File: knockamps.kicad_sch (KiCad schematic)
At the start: 6 parts, among them M6001 Module-knock-0.2, M6002 Module-knock-0.2, U6001 MCP6002-xSN

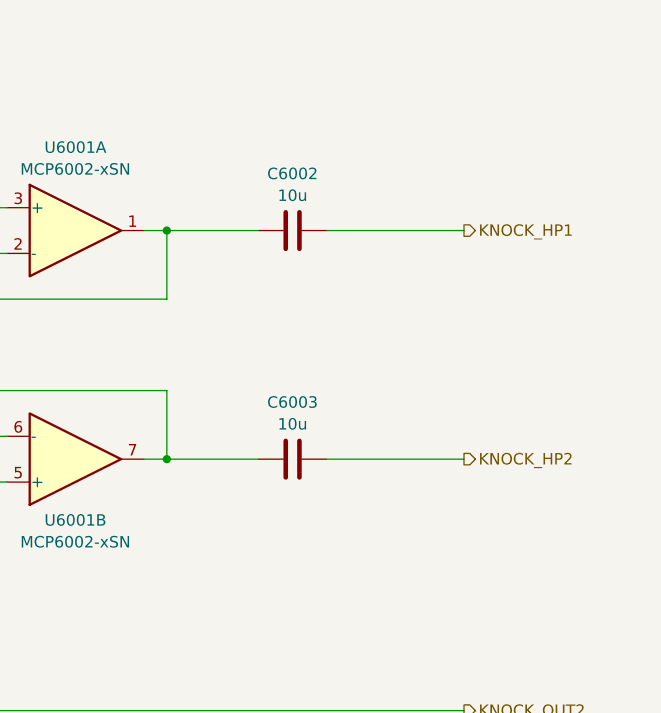
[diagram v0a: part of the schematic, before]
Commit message: Initial schematic
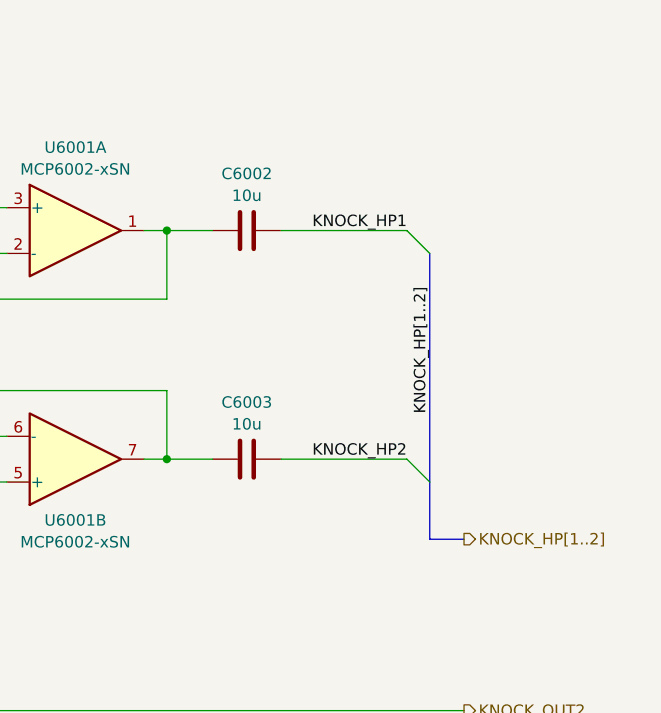
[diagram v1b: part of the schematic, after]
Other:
- moved on the sheet: C6002, C6003
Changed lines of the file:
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@@
+		)
+	)
+	(bus_entry
+		(at 240.03 99.06)
+		(size 2.54 2.54)
+		(stroke
+			(width 0)
+			(type default)
+		)
+	)
+	(bus_entry
+		(at 240.03 73.66)
+		(size 2.54 2.54)
+		(stroke
+			(width 0)
+			(type default)
 		)
 	)
@@
 	(wire
 		(pts
-			(xy 213.36 99.06) (xy 223.52 99.06)
+			(xy 213.36 99.06) (xy 218.44 99.06)
 		)
 		(stroke
@@
 	(wire
 		(pts
+			(xy 226.06 73.66) (xy 240.03 73.66)
+		)
+		(stroke
+			(width 0)
+			(type default)
+		)
+	)
+	(wire
+		(pts
 			(xy 138.43 97.79) (xy 138.43 21.59)
 		)
@@
 	(wire
 		(pts
-			(xy 231.14 99.06) (xy 246.38 99.06)
-		)
-		(stroke
-			(width 0)
-			(type default)
-		)
-	)
-	(wire
-		(pts
 			(xy 58.42 45.72) (xy 72.39 45.72)
 		)
@@
 		)
 	)
-	(wire
-		(pts
-			(xy 231.14 73.66) (xy 246.38 73.66)
+	(bus
+		(pts
+			(xy 246.38 107.95) (xy 242.57 107.95)
 		)
 		(stroke
@@
 		)
 	)
+	(bus
+		(pts
+			(xy 242.57 76.2) (xy 242.57 101.6)
+		)
+		(stroke
+			(width 0)
+			(type default)
+		)
+	)
 	(wire
 		(pts
@@
 	(wire
 		(pts
+			(xy 226.06 99.06) (xy 240.03 99.06)
+		)
+		(stroke
+			(width 0)
+			(type default)
+		)
+	)
+	(wire
+		(pts
 			(xy 153.67 76.2) (xy 163.83 76.2)
 		)
@@
 		)
 	)
+	(bus
+		(pts
+			(xy 242.57 107.95) (xy 242.57 101.6)
+		)
+		(stroke
+			(width 0)
+			(type default)
+		)
+	)
 	(wire
 		(pts
@@
 	(wire
 		(pts
-			(xy 213.36 73.66) (xy 223.52 73.66)
+			(xy 213.36 73.66) (xy 218.44 73.66)
 		)
 		(stroke
@@
 			(width 0)
 			(type default)
+		)
+	)
+	(label "KNOCK_HP1"
+		(at 240.03 73.66 180)
+		(effects
+			(font
+				(size 1.27 1.27)
+			)
+			(justify right bottom)
 		)
 	)
@@
 		)
 	)
+	(label "KNOCK_HP2"
+		(at 240.03 99.06 180)
+		(effects
+			(font
+				(size 1.27 1.27)
+			)
+			(justify right bottom)
+		)
+	)
 	(label "KNOCK1"
 		(at 60.96 45.72 0)
+		(effects
+			(font
+				(size 1.27 1.27)
+			)
+			(justify left bottom)
+		)
+	)
+	(label "KNOCK_HP[1..2]"
+		(at 242.57 93.98 90)
 		(effects
 			(font
@@
 		)
 	)
-	(hierarchical_label "KNOCK_HP1"
+	(hierarchical_label "KNOCK_HP[1..2]"
 		(shape output)
-		(at 246.38 73.66 0)
+		(at 246.38 107.95 0)
 		(effects
 			(font
@@
 		(shape output)
 		(at 246.38 45.72 0)
-		(effects
-			(font
-				(size 1.27 1.27)
-			)
-			(justify left)
-		)
-	)
-	(hierarchical_label "KNOCK_HP2"
-		(shape output)
-		(at 246.38 99.06 0)
 		(effects
 			(font
@@
 	(symbol
 		(lib_id "Device:C")
-		(at 227.33 73.66 90)
+		(at 222.25 73.66 90)
 		(unit 1)
 		(exclude_from_sim no)
@@
 		(fields_autoplaced yes)
 		(property "Reference" "C6002"
-			(at 227.33 67.3565 90)
+			(at 222.25 67.3565 90)
 			(effects
 				(font
@@
 		)
 		(property "Value" "10u"
-			(at 227.33 69.7808 90)
+			(at 222.25 69.7808 90)
 			(effects
 				(font
@@
 		)
 		(property "Footprint" "Capacitor_SMD:C_0603_1608Metric"
-			(at 231.14 72.6948 0)
+			(at 226.06 72.6948 0)
 			(effects
 				(font
@@
 		)
 		(property "Datasheet" "~"
-			(at 227.33 73.66 0)
+			(at 222.25 73.66 0)
 			(effects
 				(font
@@
 		)
 		(property "Description" "Unpolarized capacitor"
-			(at 227.33 73.66 0)
+			(at 222.25 73.66 0)
 			(effects
 				(font
@@
 	(symbol
 		(lib_id "Device:C")
-		(at 227.33 99.06 90)
+		(at 222.25 99.06 90)
 		(unit 1)
 		(exclude_from_sim no)
@@
 		(fields_autoplaced yes)
 		(property "Reference" "C6003"
-			(at 227.33 92.7565 90)
+			(at 222.25 92.7565 90)
 			(effects
 				(font
@@
 		)
 		(property "Value" "10u"
-			(at 227.33 95.1808 90)
+			(at 222.25 95.1808 90)
 			(effects
 				(font
@@
 		)
 		(property "Footprint" "Capacitor_SMD:C_0603_1608Metric"
-			(at 231.14 98.0948 0)
+			(at 226.06 98.0948 0)
 			(effects
 				(font
@@
 		)
 		(property "Datasheet" "~"
-			(at 227.33 99.06 0)
+			(at 222.25 99.06 0)
 			(effects
 				(font
@@
 		)
 		(property "Description" "Unpolarized capacitor"
-			(at 227.33 99.06 0)
-			(effects
-				(font
+			(at 222.25 99.06 0)
+			(effects
+				(font

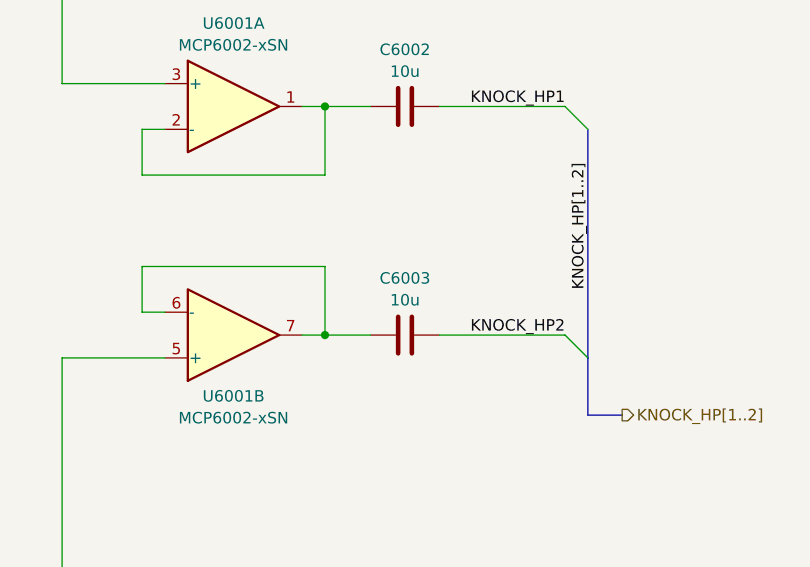
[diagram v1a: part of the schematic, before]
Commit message: adjusted BOM
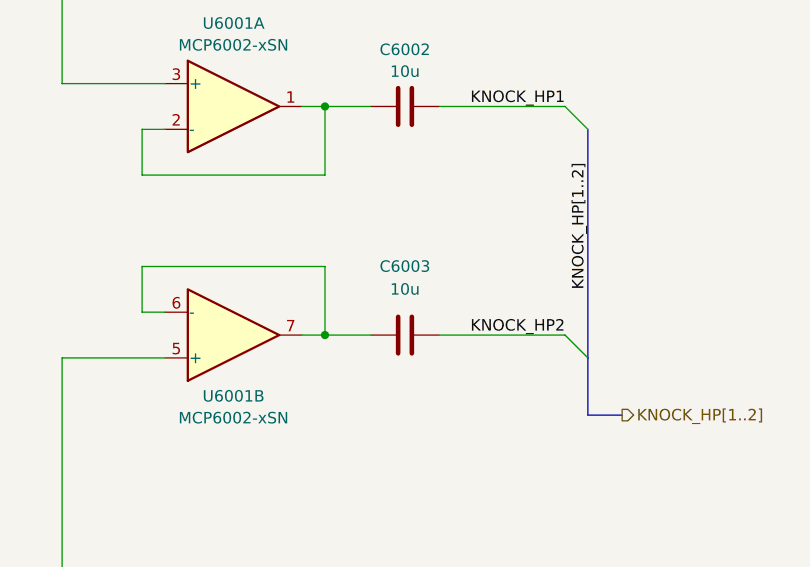
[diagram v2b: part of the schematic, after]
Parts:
- C6001: footprint Capacitor_SMD:C_0603_1608Metric -> hellen-one-common:C0805; LCSC (none) -> C597285
- C6002, C6003: footprint Capacitor_SMD:C_0603_1608Metric -> hellen-one-common:C0805; LCSC (none) -> C440198
- U6001: LCSC (none) -> C636235
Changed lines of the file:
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@@
+			)
+		)
+		(property "LCSC" "C636235"
+			(at 166.37 86.36 0)
+			(effects
+				(font
+					(size 1.27 1.27)
+				)
+				(hide yes)
 			)
 		)
@@
 			)
 		)
-		(property "Footprint" "Capacitor_SMD:C_0603_1608Metric"
+		(property "Footprint" "hellen-one-common:C0805"
 			(at 154.6352 90.17 0)
 			(effects
@@
 			)
 		)
+		(property "LCSC" "C597285"
+			(at 153.67 86.36 0)
+			(effects
+				(font
+					(size 1.27 1.27)
+				)
+				(hide yes)
+			)
+		)
 		(pin "1"
 		)
@@
 			)
 		)
-		(property "Footprint" "Capacitor_SMD:C_0603_1608Metric"
+		(property "Footprint" "hellen-one-common:C0805"
 			(at 226.06 72.6948 0)
 			(effects
@@
 			)
 		)
+		(property "LCSC" "C440198"
+			(at 222.25 73.66 0)
+			(effects
+				(font
+					(size 1.27 1.27)
+				)
+				(hide yes)
+			)
+		)
 		(pin "1"
 		)
@@
 		(fields_autoplaced yes)
 		(property "Reference" "C6003"
-			(at 222.25 92.7565 90)
+			(at 222.25 91.44 90)
 			(effects
 				(font
@@
 		)
 		(property "Value" "10u"
-			(at 222.25 95.1808 90)
-			(effects
-				(font
-					(size 1.27 1.27)
-				)
-			)
-		)
-		(property "Footprint" "Capacitor_SMD:C_0603_1608Metric"
+			(at 222.25 93.98 90)
+			(effects
+				(font
+					(size 1.27 1.27)
+				)
+			)
+		)
+		(property "Footprint" "hellen-one-common:C0805"
 			(at 226.06 98.0948 0)
 			(effects
@@
 			)
 		)
+		(property "LCSC" "C440198"
+			(at 222.25 99.06 0)
+			(effects
+				(font
+					(size 1.27 1.27)
+				)
+				(hide yes)
+			)
+		)
 		(pin "1"
 		)
@@
 		)
 		(property "Description" "1MHz, Low-Power Op Amp, SOIC-8"
+			(at 203.2 73.66 0)
+			(effects
+				(font
+					(size 1.27 1.27)
+				)
+				(hide yes)
+			)
+		)
+		(property "LCSC" "C636235"
 			(at 203.2 73.66 0)
 			(effects
@@
 			(at 203.2 99.06 0)
 			(effects
+				(font
+					(size 1.27 1.27)
+				)
+				(hide yes)
+			)
+		)
+		(property "LCSC" "C636235"
+			(at 203.2 99.06 0)
+			(effects
